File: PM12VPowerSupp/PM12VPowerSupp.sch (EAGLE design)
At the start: 29 parts

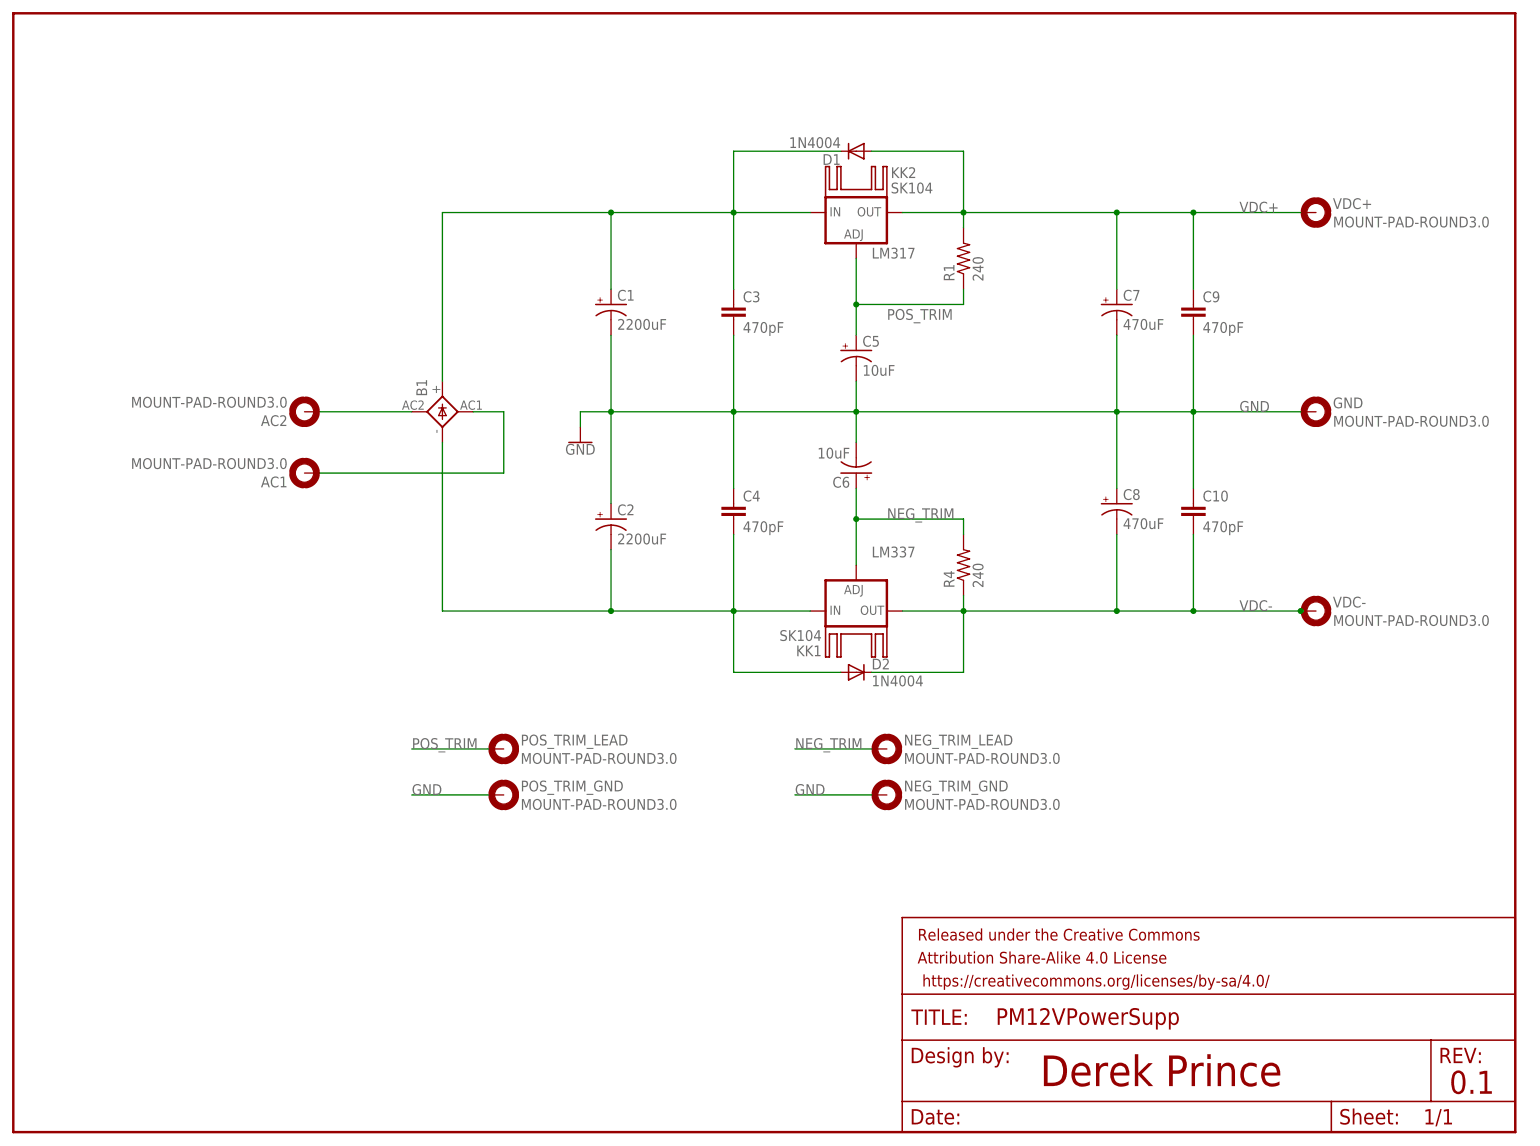
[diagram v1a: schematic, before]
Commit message: Revert "No more air wires. Have to do relief holes and heat sinks"
This reverts commit 0472ab177aecc554d98bdcb29c09631f317f4fda.
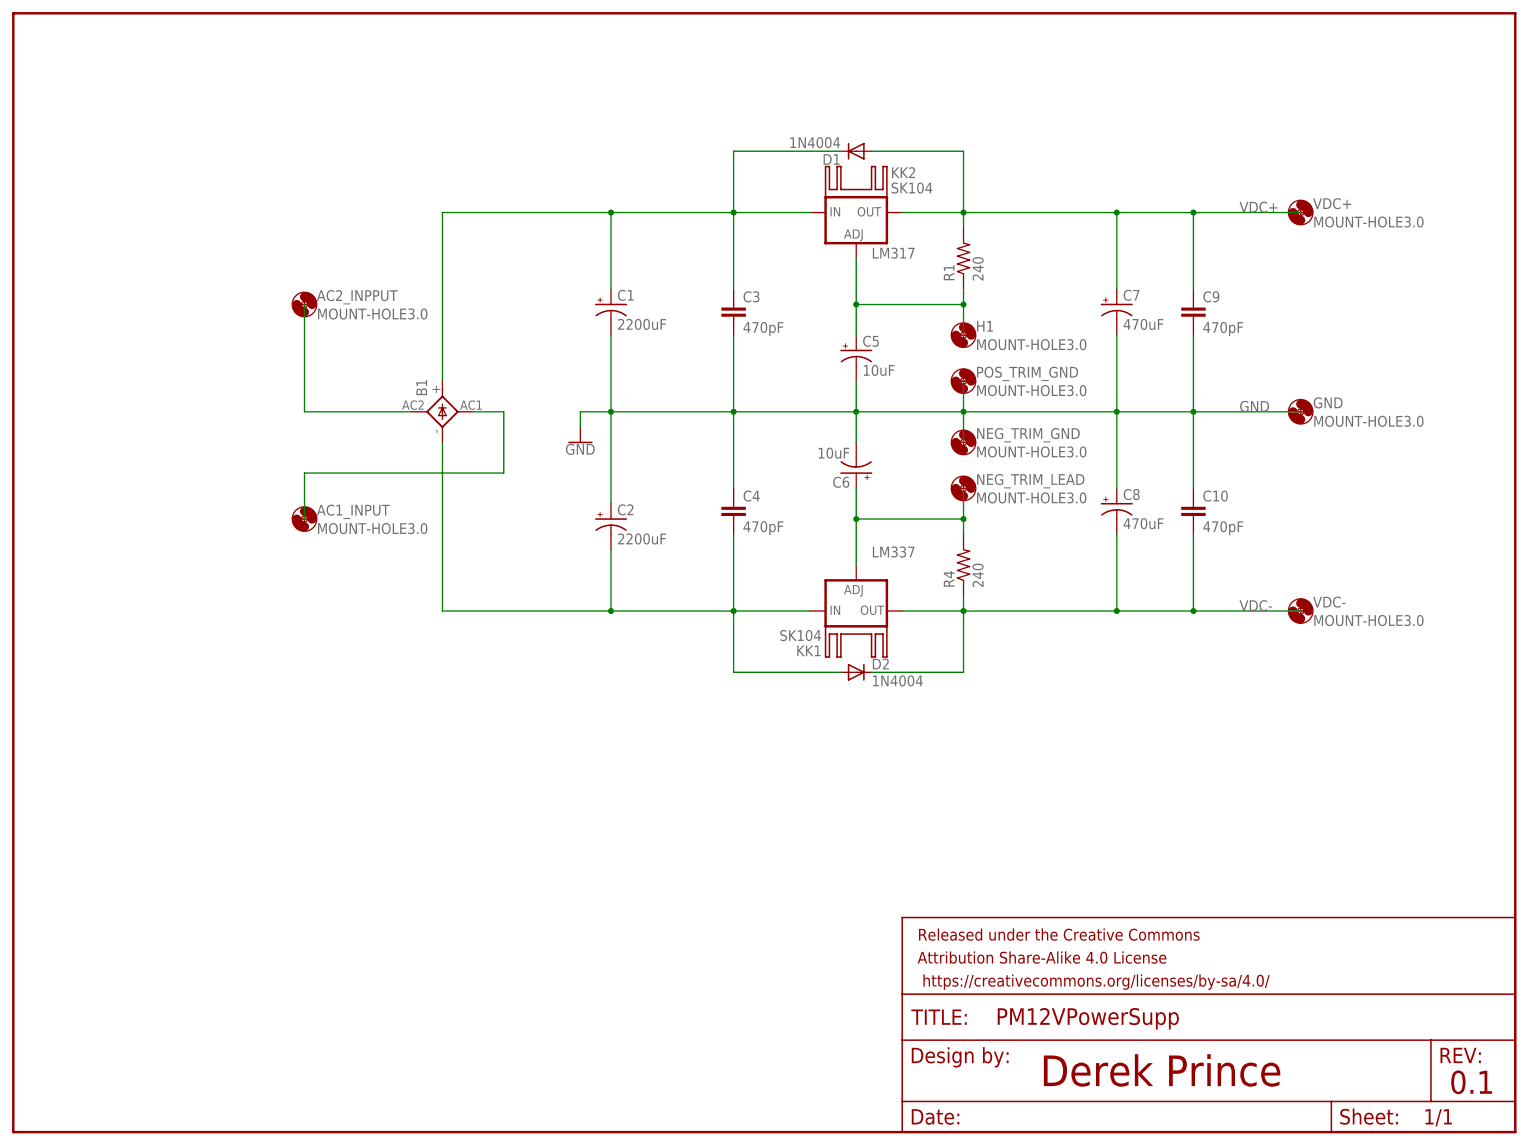
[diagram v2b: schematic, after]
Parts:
- removed AC1, AC2, POS_TRIM_LEAD: MOUNT-PAD-ROUND3.0, holes:MOUNT-PAD-ROUND3.0
- added AC1_INPUT, AC2_INPPUT, H1: MOUNT-HOLE3.0, holes:MOUNT-HOLE3.0
- GND, NEG_TRIM_GND, NEG_TRIM_LEAD, POS_TRIM_GND, VDC+, VDC-: value MOUNT-PAD-ROUND3.0 -> MOUNT-HOLE3.0; device holes:MOUNT-PAD-ROUND3.0 -> holes:MOUNT-HOLE3.0
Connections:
- removed net AC1_INPUT: AC1.MOUNT, B1.AC2
- removed net NEG_TRIM: C6.+, LM337.ADJ, NEG_TRIM_LEAD.MOUNT, R4.2
- removed net POS_TRIM: C5.+, LM317.ADJ, POS_TRIM_LEAD.MOUNT, R1.1
- new net N$2: C6.+, LM337.ADJ, R4.2
- new net N$3: B1.AC1
- new net POS_TRIM_LEAD: C5.+, LM317.ADJ, R1.1
- net GND: no longer GND.MOUNT, NEG_TRIM_GND.MOUNT, POS_TRIM_GND.MOUNT
- net N$1: now also B1.AC2; no longer AC2.MOUNT, B1.AC1
- net VDC+: no longer VDC+.MOUNT
- net VDC-: no longer VDC-.MOUNT
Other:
- moved on the sheet: GND, NEG_TRIM_GND, NEG_TRIM_LEAD, POS_TRIM_GND, VDC+, VDC-
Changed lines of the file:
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@@
 <part name="KK1" library="heatsink" deviceset="SK104" device=""/>
 <part name="KK2" library="heatsink" deviceset="SK104" device=""/>
-<part name="AC2" library="holes" deviceset="MOUNT-PAD-ROUND" device="3.0"/>
-<part name="AC1" library="holes" deviceset="MOUNT-PAD-ROUND" device="3.0"/>
-<part name="NEG_TRIM_GND" library="holes" deviceset="MOUNT-PAD-ROUND" device="3.0"/>
-<part name="NEG_TRIM_LEAD" library="holes" deviceset="MOUNT-PAD-ROUND" device="3.0"/>
-<part name="POS_TRIM_LEAD" library="holes" deviceset="MOUNT-PAD-ROUND" device="3.0"/>
-<part name="POS_TRIM_GND" library="holes" deviceset="MOUNT-PAD-ROUND" device="3.0"/>
-<part name="VDC+" library="holes" deviceset="MOUNT-PAD-ROUND" device="3.0"/>
-<part name="GND" library="holes" deviceset="MOUNT-PAD-ROUND" device="3.0"/>
-<part name="VDC-" library="holes" deviceset="MOUNT-PAD-ROUND" device="3.0"/>
+<part name="AC2_INPPUT" library="holes" deviceset="MOUNT-HOLE" device="3.0"/>
+<part name="AC1_INPUT" library="holes" deviceset="MOUNT-HOLE" device="3.0"/>
+<part name="VDC-" library="holes" deviceset="MOUNT-HOLE" device="3.0"/>
+<part name="GND" library="holes" deviceset="MOUNT-HOLE" device="3.0"/>
+<part name="VDC+" library="holes" deviceset="MOUNT-HOLE" device="3.0"/>
+<part name="H1" library="holes" deviceset="MOUNT-HOLE" device="3.0"/>
+<part name="POS_TRIM_GND" library="holes" deviceset="MOUNT-HOLE" device="3.0"/>
+<part name="NEG_TRIM_GND" library="holes" deviceset="MOUNT-HOLE" device="3.0"/>
+<part name="NEG_TRIM_LEAD" library="holes" deviceset="MOUNT-HOLE" device="3.0"/>
 </parts>
 <sheets>
@@
 <instance part="KK1" gate="1" x="139.7" y="83.82" rot="R180"/>
 <instance part="KK2" gate="1" x="139.7" y="154.94"/>
-<instance part="AC2" gate="G$1" x="48.26" y="119.38" rot="R180"/>
-<instance part="AC1" gate="G$1" x="48.26" y="109.22" rot="R180"/>
-<instance part="NEG_TRIM_GND" gate="G$1" x="144.78" y="55.88"/>
-<instance part="NEG_TRIM_LEAD" gate="G$1" x="144.78" y="63.5"/>
-<instance part="POS_TRIM_LEAD" gate="G$1" x="81.28" y="63.5"/>
-<instance part="POS_TRIM_GND" gate="G$1" x="81.28" y="55.88"/>
-<instance part="VDC+" gate="G$1" x="215.9" y="152.4"/>
-<instance part="GND" gate="G$1" x="215.9" y="119.38"/>
-<instance part="VDC-" gate="G$1" x="215.9" y="86.36"/>
+<instance part="AC2_INPPUT" gate="G$1" x="48.26" y="137.16"/>
+<instance part="AC1_INPUT" gate="G$1" x="48.26" y="101.6"/>
+<instance part="VDC-" gate="G$1" x="213.36" y="86.36"/>
+<instance part="GND" gate="G$1" x="213.36" y="119.38"/>
+<instance part="VDC+" gate="G$1" x="213.36" y="152.4"/>
+<instance part="H1" gate="G$1" x="157.48" y="132.08"/>
+<instance part="POS_TRIM_GND" gate="G$1" x="157.48" y="124.46"/>
+<instance part="NEG_TRIM_GND" gate="G$1" x="157.48" y="114.3"/>
+<instance part="NEG_TRIM_LEAD" gate="G$1" x="157.48" y="106.68"/>
 </instances>
 <busses>
 </busses>
 <nets>
-<net name="NEG_TRIM" class="0">
+<net name="N$2" class="0">
 <segment>
 <pinref part="LM337" gate="1" pin="ADJ"/>
@@
 <wire x1="157.48" y1="101.6" x2="139.7" y2="101.6" width="0.1524" layer="91"/>
 <junction x="139.7" y="101.6"/>
-<label x="144.78" y="101.6" size="1.778" layer="95"/>
-</segment>
-<segment>
-<pinref part="NEG_TRIM_LEAD" gate="G$1" pin="MOUNT"/>
-<wire x1="142.24" y1="63.5" x2="129.54" y2="63.5" width="0.1524" layer="91"/>
-<label x="129.54" y="63.5" size="1.778" layer="95"/>
-</segment>
-</net>
-<net name="POS_TRIM" class="0">
+<wire x1="157.48" y1="101.6" x2="157.48" y2="106.68" width="0.1524" layer="91"/>
+<junction x="157.48" y="101.6"/>
+</segment>
+</net>
+<net name="POS_TRIM_LEAD" class="0">
 <segment>
 <pinref part="LM317" gate="1" pin="ADJ"/>
@@
 <pinref part="R1" gate="G$1" pin="1"/>
 <wire x1="157.48" y1="137.16" x2="157.48" y2="139.7" width="0.1524" layer="91"/>
-<label x="144.78" y="134.62" size="1.778" layer="95"/>
-</segment>
-<segment>
-<pinref part="POS_TRIM_LEAD" gate="G$1" pin="MOUNT"/>
-<wire x1="78.74" y1="63.5" x2="66.04" y2="63.5" width="0.1524" layer="91"/>
-<label x="66.04" y="63.5" size="1.778" layer="95"/>
+<wire x1="157.48" y1="132.08" x2="157.48" y2="137.16" width="0.1524" layer="91"/>
+<junction x="157.48" y="137.16"/>
 </segment>
 </net>
@@
 <junction x="195.58" y="152.4"/>
 <label x="203.2" y="152.4" size="1.778" layer="95"/>
-<pinref part="VDC+" gate="G$1" pin="MOUNT"/>
 </segment>
 </net>
@@
 <wire x1="157.48" y1="76.2" x2="157.48" y2="86.36" width="0.1524" layer="91"/>
 <label x="203.2" y="86.36" size="1.778" layer="95"/>
-<pinref part="VDC-" gate="G$1" pin="MOUNT"/>
-<junction x="213.36" y="86.36"/>
 </segment>
 </net>
@@
 <wire x1="99.06" y1="119.38" x2="119.38" y2="119.38" width="0.1524" layer="91"/>
 <wire x1="119.38" y1="119.38" x2="139.7" y2="119.38" width="0.1524" layer="91"/>
-<wire x1="139.7" y1="119.38" x2="182.88" y2="119.38" width="0.1524" layer="91"/>
+<wire x1="139.7" y1="119.38" x2="157.48" y2="119.38" width="0.1524" layer="91"/>
+<wire x1="157.48" y1="119.38" x2="182.88" y2="119.38" width="0.1524" layer="91"/>
 <wire x1="182.88" y1="119.38" x2="195.58" y2="119.38" width="0.1524" layer="91"/>
 <wire x1="99.06" y1="104.14" x2="99.06" y2="119.38" width="0.1524" layer="91"/>
@@
 <wire x1="195.58" y1="119.38" x2="213.36" y2="119.38" width="0.1524" layer="91"/>
 <label x="203.2" y="119.38" size="1.778" layer="95"/>
-<pinref part="GND" gate="G$1" pin="MOUNT"/>
-</segment>
-<segment>
-<pinref part="NEG_TRIM_GND" gate="G$1" pin="MOUNT"/>
-<wire x1="142.24" y1="55.88" x2="129.54" y2="55.88" width="0.1524" layer="91"/>
-<label x="129.54" y="55.88" size="1.778" layer="95"/>
-</segment>
-<segment>
-<pinref part="POS_TRIM_GND" gate="G$1" pin="MOUNT"/>
-<wire x1="78.74" y1="55.88" x2="66.04" y2="55.88" width="0.1524" layer="91"/>
-<label x="66.04" y="55.88" size="1.778" layer="95"/>
-</segment>
-</net>
-<net name="AC1_INPUT" class="0">
+<junction x="157.48" y="119.38"/>
+<wire x1="157.48" y1="124.46" x2="157.48" y2="119.38" width="0.1524" layer="91"/>
+<wire x1="157.48" y1="114.3" x2="157.48" y2="119.38" width="0.1524" layer="91"/>
+</segment>
+</net>
+<net name="N$1" class="0">
 <segment>
 <pinref part="B1" gate="1" pin="AC2"/>
 <wire x1="76.2" y1="119.38" x2="81.28" y2="119.38" width="0.1524" layer="91"/>
 <wire x1="81.28" y1="119.38" x2="81.28" y2="109.22" width="0.1524" layer="91"/>
-<wire x1="81.28" y1="109.22" x2="50.8" y2="109.22" width="0.1524" layer="91"/>
-<pinref part="AC1" gate="G$1" pin="MOUNT"/>
-</segment>
-</net>
-<net name="N$1" class="0">
+<wire x1="81.28" y1="109.22" x2="48.26" y2="109.22" width="0.1524" layer="91"/>
+<wire x1="48.26" y1="109.22" x2="48.26" y2="101.6" width="0.1524" layer="91"/>
+</segment>
+</net>
+<net name="N$3" class="0">
 <segment>
 <pinref part="B1" gate="1" pin="AC1"/>
-<pinref part="AC2" gate="G$1" pin="MOUNT"/>
-<wire x1="50.8" y1="119.38" x2="66.04" y2="119.38" width="0.1524" layer="91"/>
+<wire x1="66.04" y1="119.38" x2="48.26" y2="119.38" width="0.1524" layer="91"/>
+<wire x1="48.26" y1="119.38" x2="48.26" y2="137.16" width="0.1524" layer="91"/>
 </segment>
 </net>
@@
 </sheet>
 </sheets>
-<errors>
-</errors>
 </schematic>
 </drawing>
